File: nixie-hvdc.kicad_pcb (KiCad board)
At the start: 2 copper layers, 66 x 66 mm, 41 parts, among them J1 Conn_01x11_Pin, J2 PJ-002B, J3 Screw_Terminal_01x02, J4 Screw_Terminal_01x02, Q1 MPSA42, Q10 MPSA42, Q11 MPSA42, Q12 IRF740, Q2 MPSA42, Q3 MPSA42, Q4 MPSA42, Q5 MPSA42, Q6 MPSA42, Q7 MPSA42, Q8 MPSA42, Q9 MPSA42, U1 MAX1771xSA

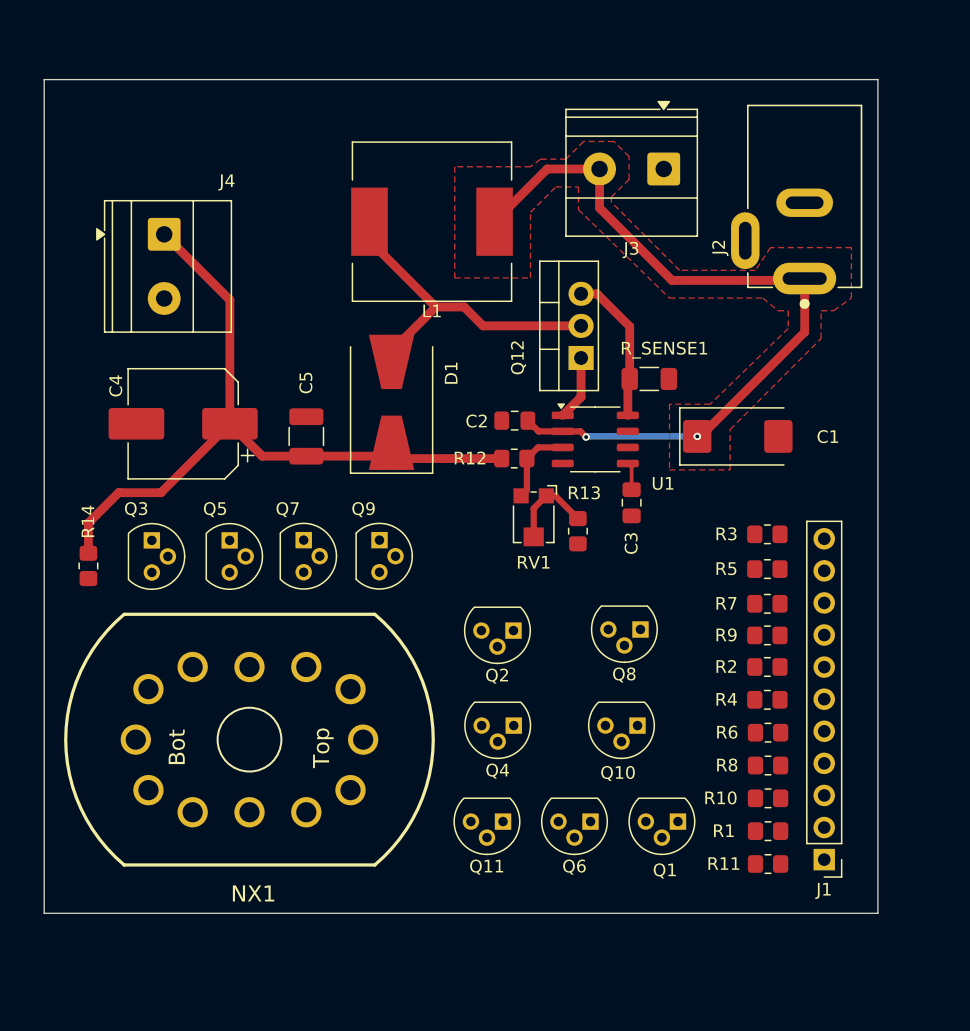
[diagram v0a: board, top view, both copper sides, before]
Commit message: nearly done?
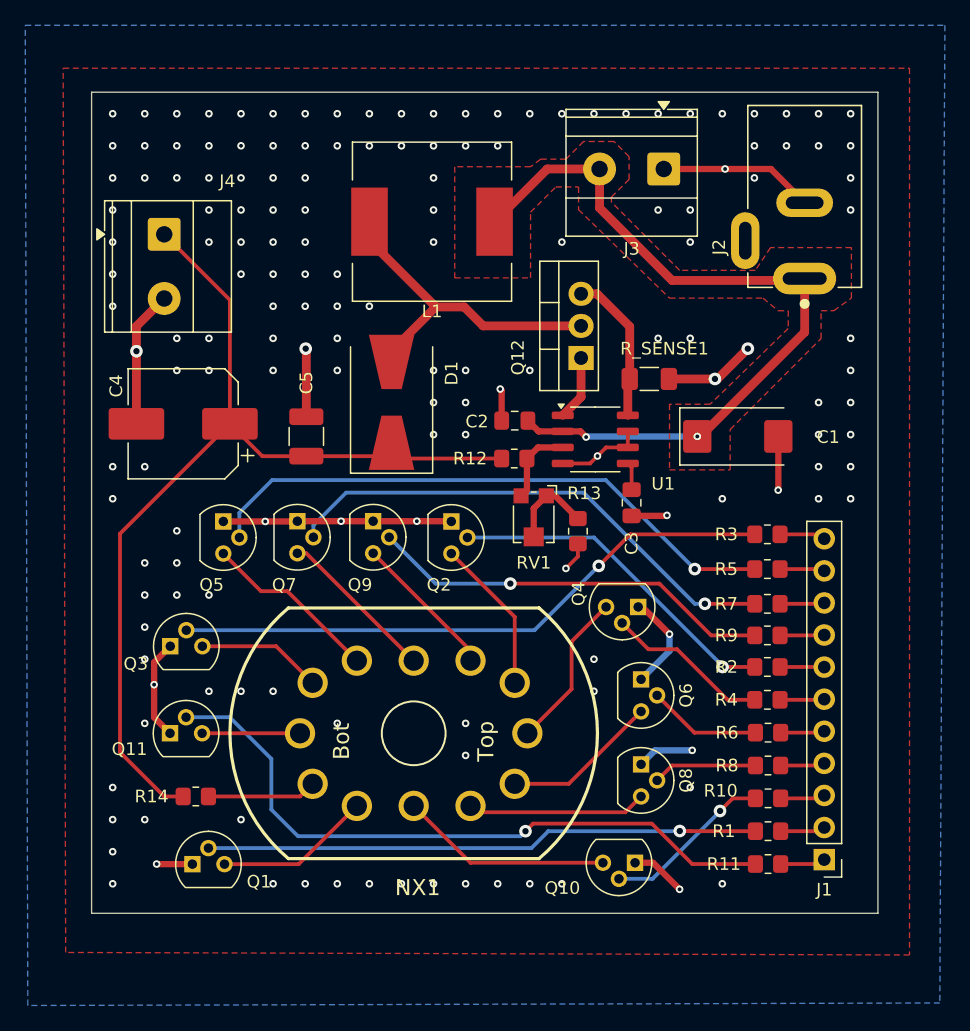
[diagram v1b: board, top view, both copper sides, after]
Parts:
- moved Q1 38.6 mm to (128.2, 122.6), turned to 0 degrees
- moved Q11 27.3 mm to (126.5, 112.2), turned to 0 degrees
- moved R14 20.1 mm to (128.5, 117.2), turned to 180 degrees
- moved Q4 13.6 mm to (163.5, 102.2)
- moved NX1 13.0 mm to (145.8, 112.2)
- moved Q6 11.9 mm to (163.8, 108.0), turned to -90 degrees
- moved Q10 10.9 mm to (163.3, 122.5)
- moved Q8 10.7 mm to (163.8, 114.7), turned to -90 degrees
- moved Q2 9.94 mm to (148.7, 95.5), turned to -90 degrees
- moved Q3 8.51 mm to (126.5, 105.4), turned to 0 degrees
- moved Q5 1.58 mm to (130.7, 95.5)
- moved Q7 1.58 mm to (136.5, 95.5)
- moved Q9 1.58 mm to (142.5, 95.5)
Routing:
- net GND: track 0.00 -> 100.3 mm, vias 0 -> 162
- net Net-(Q11-B): track 0.00 -> 53.1 mm, vias 0 -> 1
- net Net-(Q3-B): track 0.00 -> 48.1 mm, vias 0 -> 1
- net Net-(Q5-B): track 0.00 -> 46.7 mm, vias 0 -> 1
- net Net-(Q1-B): track 0.00 -> 43.9 mm, vias 0 -> 1
- net Net-(Q7-B): track 0.00 -> 40.6 mm, vias 0 -> 1
- net Net-(Q9-B): track 0.00 -> 32.2 mm, vias 0 -> 1
- net Net-(Q2-B): track 0.00 -> 27.0 mm, vias 0 -> 1
- net /180V: track 57.5 -> 76.7 mm
- net /NIXIE_DIGIT_9: track 0.00 -> 16.8 mm
- net /NIXIE_DIGIT_8: track 0.00 -> 14.2 mm
- net /NIXIE_DIGIT_2: track 0.00 -> 14.1 mm
- net Net-(Q10-B): track 0.00 -> 13.5 mm, vias 0 -> 1
- net Net-(Q4-B): track 0.00 -> 13.0 mm
- net /NIXIE_DIGIT_3: track 0.00 -> 12.8 mm
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- added copper zone on B.Cu, net GND
- added copper zone on F.Cu, net GND
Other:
- board size 66 x 66 mm -> 62.2 x 65 mm
- board text added: "{ "ViaStitching": "0.2", "SWITCHING_STITCHING_VIAS": { "HSpacing": "1", "VSpacing": "1", "HOffset": "0", "VOffset": "0", "Clearance": "0", "Randomize": false } }"
- board text added: "{ "ViaStitching": "0.2", "SWITCHING_STITCHING_VIAS": { "HSpacing": "3", "VSpacing": "3", "HOffset": "0", "VOffset": "0", "Clearance": "0", "Randomize": false } }"
- board text added: "{ "ViaStitching": "0.2", "SWITCHING_STITCHING_VIAS": { "HSpacing": "7", "VSpacing": "7", "HOffset": "0", "VOffset": "0", "Clearance": "0", "Randomize": false } }"
- board text added: "{ "ViaStitching": "0.2", "SWITCHING_STITCHING_VIAS": { "HSpacing": "7", "VSpacing": "7", "HOffset": "0", "VOffset": "0", "Clearance": "3", "Randomize": false } }"
- board text added: "{ "ViaStitching": "0.2", "SWITCHING_STITCHING_VIAS": { "HSpacing": "7", "VSpacing": "7", "HOffset": "0", "VOffset": "0", "Clearance": "5", "Randomize": false } }"
- board text added: "{ "ViaStitching": "0.2", "stitch_zone_0": { "HSpacing": "1", "VSpacing": "1", "HOffset": "0", "VOffset": "0", "Clearance": "0", "Randomize": false } }"
- board text added: "{ "ViaStitching": "0.2", "stitch_zone_0": { "HSpacing": "3", "VSpacing": "3", "HOffset": "0.5", "VOffset": "1", "Clearance": "0", "Randomize": false } }"
